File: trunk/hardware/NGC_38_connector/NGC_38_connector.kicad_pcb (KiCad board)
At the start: 2 copper layers, 38 x 29 mm, 5 parts, among them P1 DIL38, P2 CONN_10, P3 CONN_9, P4 CONN_10, P5 CONN_9

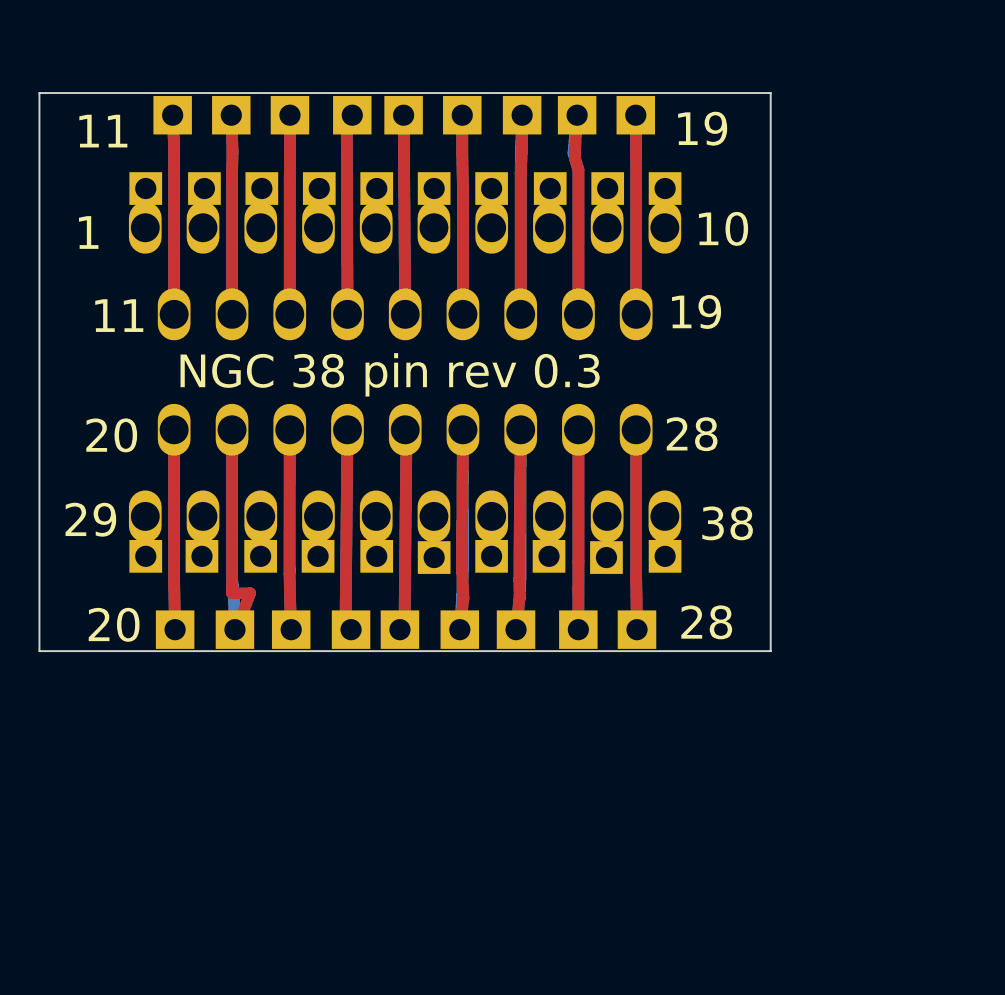
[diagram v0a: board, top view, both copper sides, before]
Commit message: 4.0.1
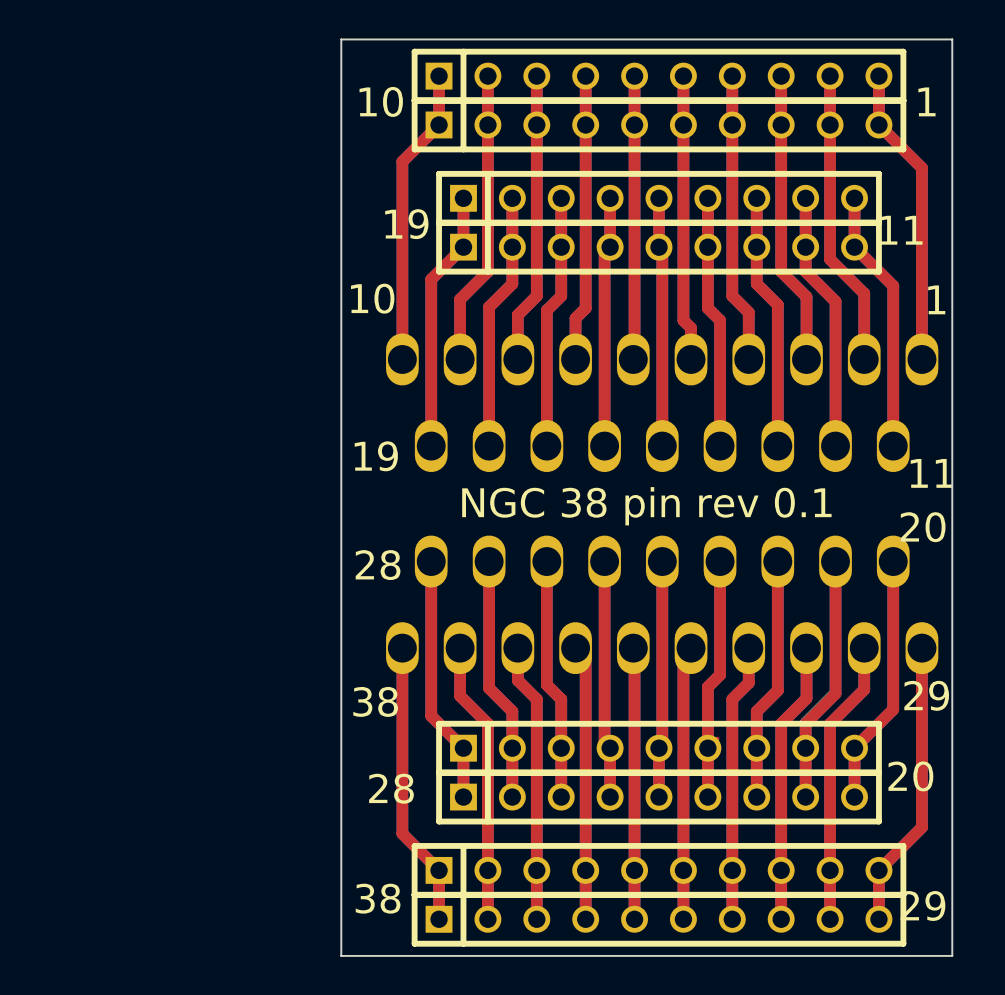
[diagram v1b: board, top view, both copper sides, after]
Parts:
- added P6: CONN_10, SIL-10, F.Cu at (163.2, 134.6)
- added P7: CONN_9, SIL-9, F.Cu at (163.2, 141.0)
- added P8: CONN_9, SIL-9, F.Cu at (163.2, 172.1)
- added P9: CONN_10, SIL-10, F.Cu at (163.2, 178.4)
- moved P4 21.4 mm to (163.2, 175.9)
- moved P3 15.1 mm to (163.2, 143.5)
- moved P1 15.0 mm to (149.9, 156.8)
- moved P5 14.8 mm to (163.2, 169.5)
- moved P2 13.9 mm to (163.2, 137.2)
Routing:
- net N-0000010: track 2.04 -> 31.3 mm
- net N-000001: track 2.05 -> 31.0 mm
- net N-000009: track 2.05 -> 30.9 mm
- net N-000002: track 2.07 -> 30.6 mm
- net N-000008: track 2.06 -> 30.5 mm
- net N-000003: track 2.06 -> 30.3 mm
- net N-000007: track 2.04 -> 30.2 mm
- net N-0000035: track 2.08 -> 30.0 mm
- net N-000004: track 2.06 -> 29.9 mm
- net N-000006: track 2.04 -> 29.8 mm
- net N-0000027: track 2.09 -> 29.8 mm
- net N-0000034: track 2.15 -> 29.7 mm
- net N-000005: track 2.05 -> 29.5 mm
- net N-0000028: track 2.10 -> 29.4 mm
- net N-0000033: track 2.08 -> 29.3 mm
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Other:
- board size 38 x 29 mm -> 31.8 x 47.6 mm
- board text added: "NGC 38 pin rev 0.1"
- board text removed: "NGC 38 pin rev 0.3"
